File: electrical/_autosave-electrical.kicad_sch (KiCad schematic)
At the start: 29 parts, among them J1 Raspberry Pi GPIO, J2 Touch screen connector, J3 Load_cell, J4 PIR_sensor, J9 Water_sensor, K1 RAYEX-L90, M1 Milk_powder, M2 Instant_coffee, M3 Sugar, M4 Motor_DC, P1 IEC_60320_C13_Plug, Q1 2N3904, Q4 2N3904, SW1 Thermostat, SW2 SW_SPDT, U1 A4988_STEPPER_MOTOR_DRIVER_CA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, U2 A4988_STEPPER_MOTOR_DRIVER_CA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, U3 A4988_STEPPER_MOTOR_DRIVER_CA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, U5 PC817

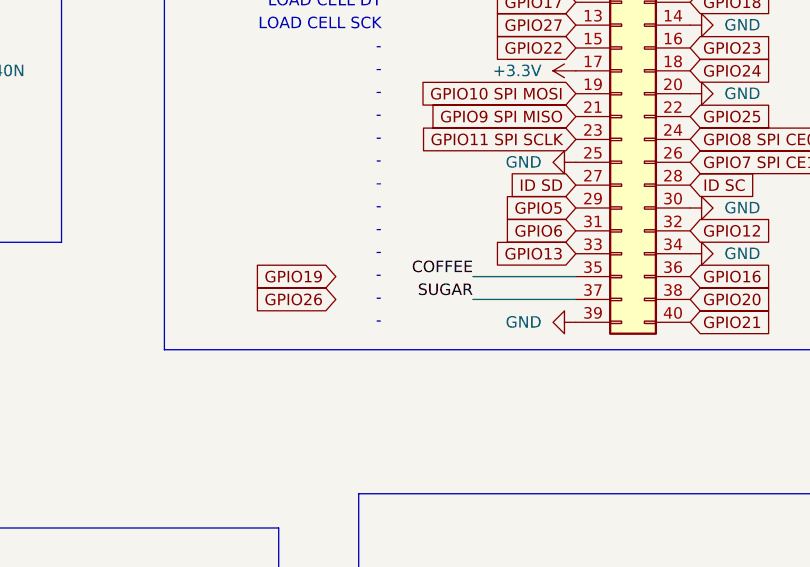
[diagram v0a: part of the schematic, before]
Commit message: first commit
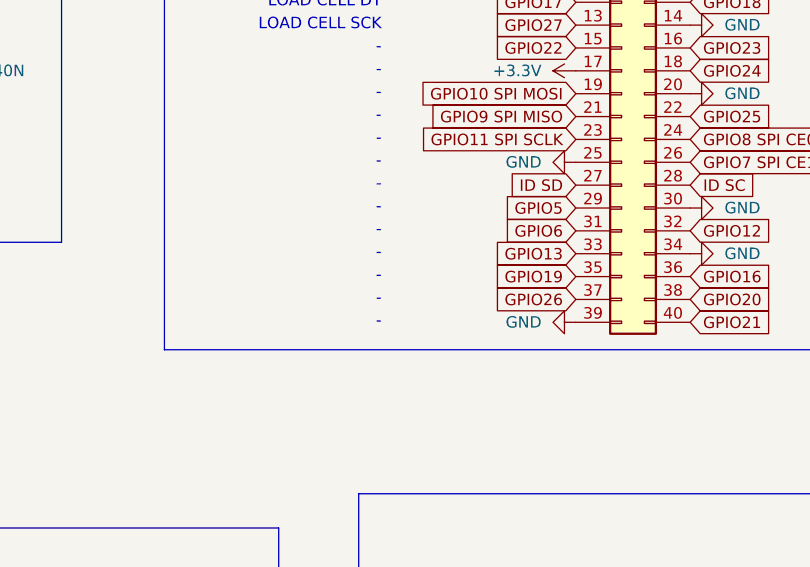
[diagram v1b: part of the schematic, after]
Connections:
- net COFFEE: no longer J1.35 (Pin_35)
- net GPIO19: now also J1.35 (Pin_35)
- net GPIO26: now also J1.37 (Pin_37)
- net SUGAR: no longer J1.37 (Pin_37)
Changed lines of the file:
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@@
-	(wire
-		(pts
-			(xy 196.85 76.2) (xy 208.28 76.2)
-		)
-		(stroke
-			(width 0)
-			(type default)
-		)
-	)
-	(wire
-		(pts
-			(xy 196.85 73.66) (xy 208.28 73.66)
-		)
-		(stroke
-			(width 0)
-			(type default)
-		)
-	)
 	(wire
 		(pts
@@
 	)
 	(label "COFFEE"
-		(at 196.85 73.66 180)
-		(fields_autoplaced yes)
-		(effects
-			(font
-				(size 1.27 1.27)
-			)
-			(justify right bottom)
-		)
-	)
-	(label "SUGAR"
-		(at 196.85 76.2 180)
-		(fields_autoplaced yes)
-		(effects
-			(font
-				(size 1.27 1.27)
-			)
-			(justify right bottom)
-		)
-	)
-	(label "COFFEE"
 		(at 40.64 76.2 0)
 		(fields_autoplaced yes)
@@
 	(global_label "GPIO19"
 		(shape input)
-		(at 181.61 73.66 180)
-		(fields_autoplaced yes)
-		(effects
-			(font
-				(size 1.27 1.27)
-			)
-			(justify right)
-		)
-		(property "Intersheetrefs" "${INTERSHEET_REFS}"
-			(at 171.7305 73.66 0)
+		(at 208.28 73.66 180)
+		(fields_autoplaced yes)
+		(effects
+			(font
+				(size 1.27 1.27)
+			)
+			(justify right)
+		)
+		(property "Intersheetrefs" "${INTERSHEET_REFS}"
+			(at 198.4005 73.66 0)
 			(effects
 				(font
@@
 	(global_label "GPIO26"
 		(shape input)
-		(at 181.61 76.2 180)
-		(fields_autoplaced yes)
-		(effects
-			(font
-				(size 1.27 1.27)
-			)
-			(justify right)
-		)
-		(property "Intersheetrefs" "${INTERSHEET_REFS}"
-			(at 171.7305 76.2 0)
-			(effects
-				(font
+		(at 208.28 76.2 180)
+		(fields_autoplaced yes)
+		(effects
+			(font
+				(size 1.27 1.27)
+			)
+			(justify right)
+		)
+		(property "Intersheetrefs" "${INTERSHEET_REFS}"
+			(at 198.4005 76.2 0)
+			(effects
+				(font
